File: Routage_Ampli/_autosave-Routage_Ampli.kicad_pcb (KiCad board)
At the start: 2 copper layers, 110.5 x 100.3 mm, 52 parts, among them J1 Conn_01x03, J2 Conn_01x02, Q1 2N2907, Q10 TIP32, Q11 BD138, Q12 TIP31, Q13 2N2222, Q2 2N2907, Q3 2N2907, Q4 2N2222, Q5 2N2222, Q6 2N2907, Q7 2N2907, Q8 BD139, Q9 BD139, U1 Jack_Mono, U2 Relay_1CT

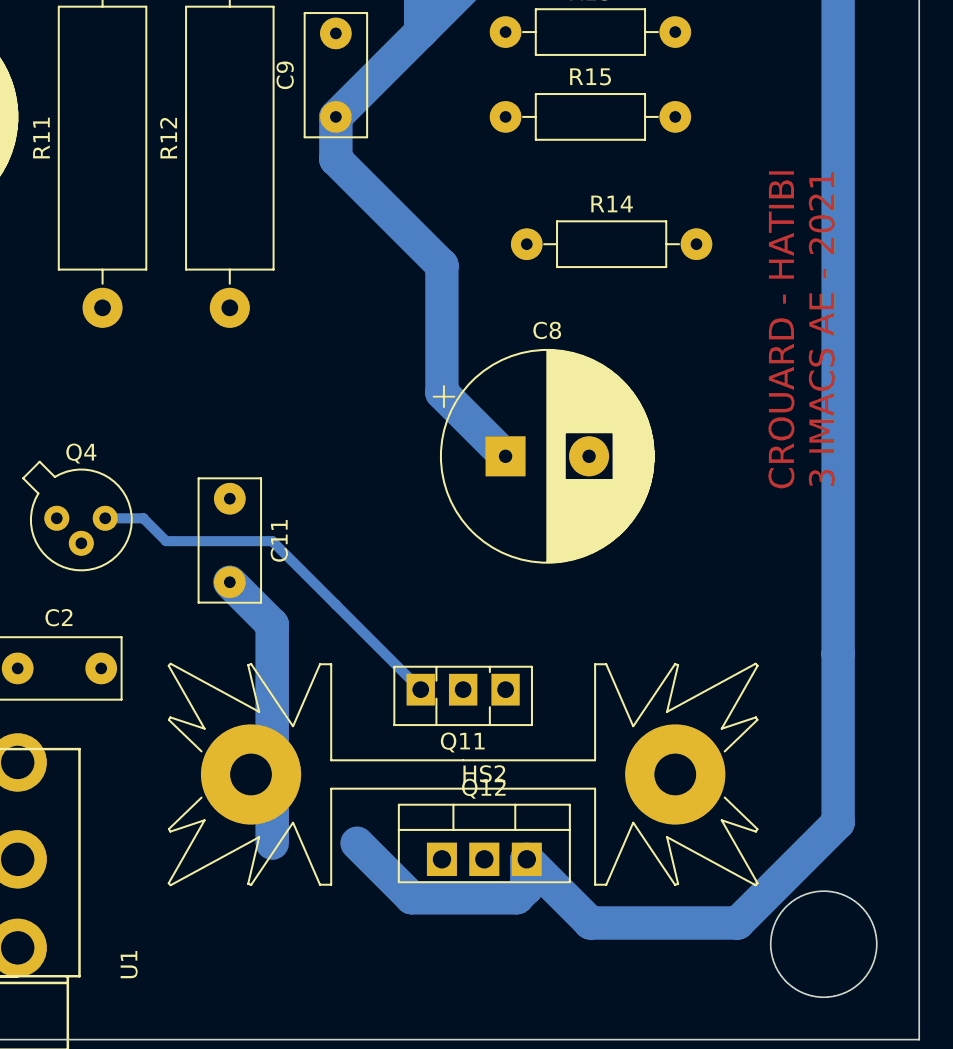
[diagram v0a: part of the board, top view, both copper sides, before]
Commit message: Version avant correction
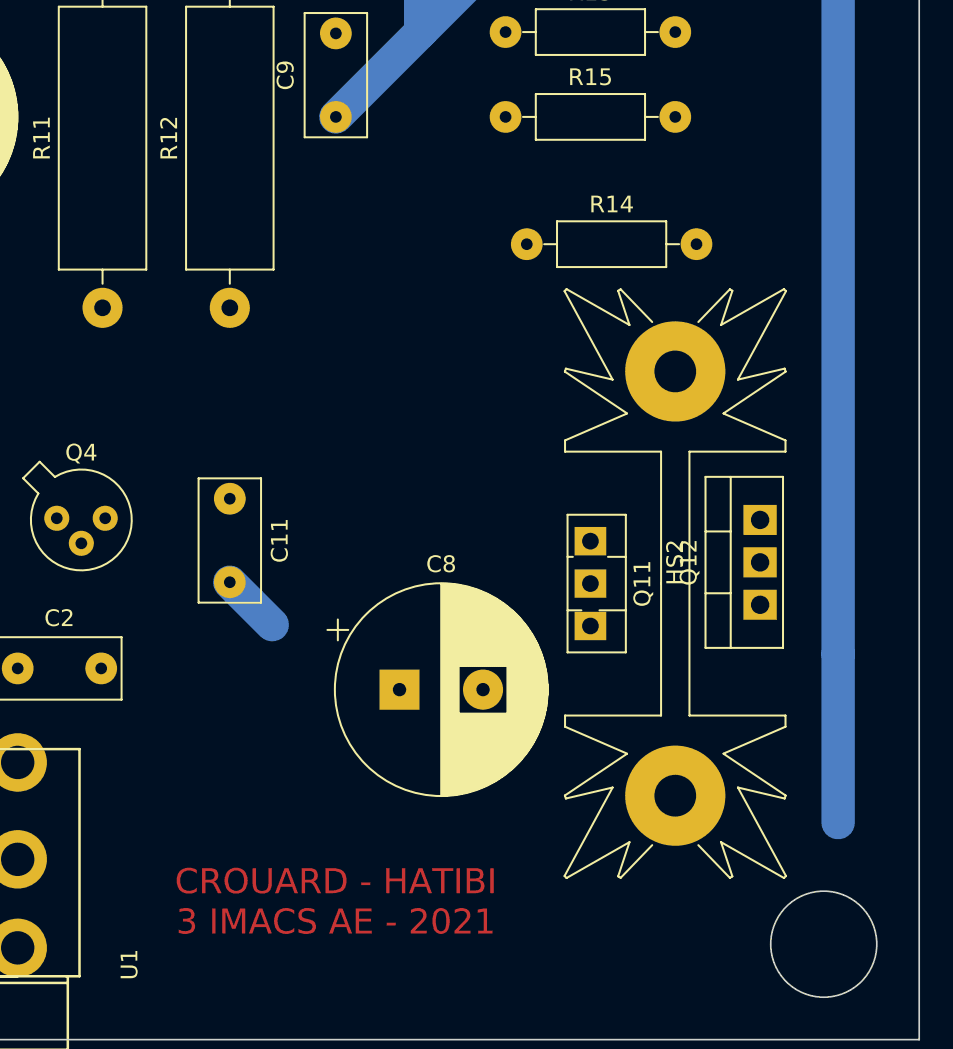
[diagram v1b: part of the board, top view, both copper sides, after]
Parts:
- moved Q12 24.4 mm to (199.4, 116.8), turned to 90 degrees
- moved HS2 17.1 mm to (194.3, 115.6), turned to 270 degrees
- moved C8 15.3 mm to (177.8, 121.9)
- moved Q11 10.2 mm to (189.2, 113.0), turned to 270 degrees
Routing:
- net -12V: track 369.4 -> 320.1 mm
- net +12V: track 199.1 -> 174.5 mm
- net Net-(C2-Pad1): track 23.1 -> 0.00 mm
